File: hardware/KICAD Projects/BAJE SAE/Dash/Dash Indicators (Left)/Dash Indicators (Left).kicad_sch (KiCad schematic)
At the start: 16 parts

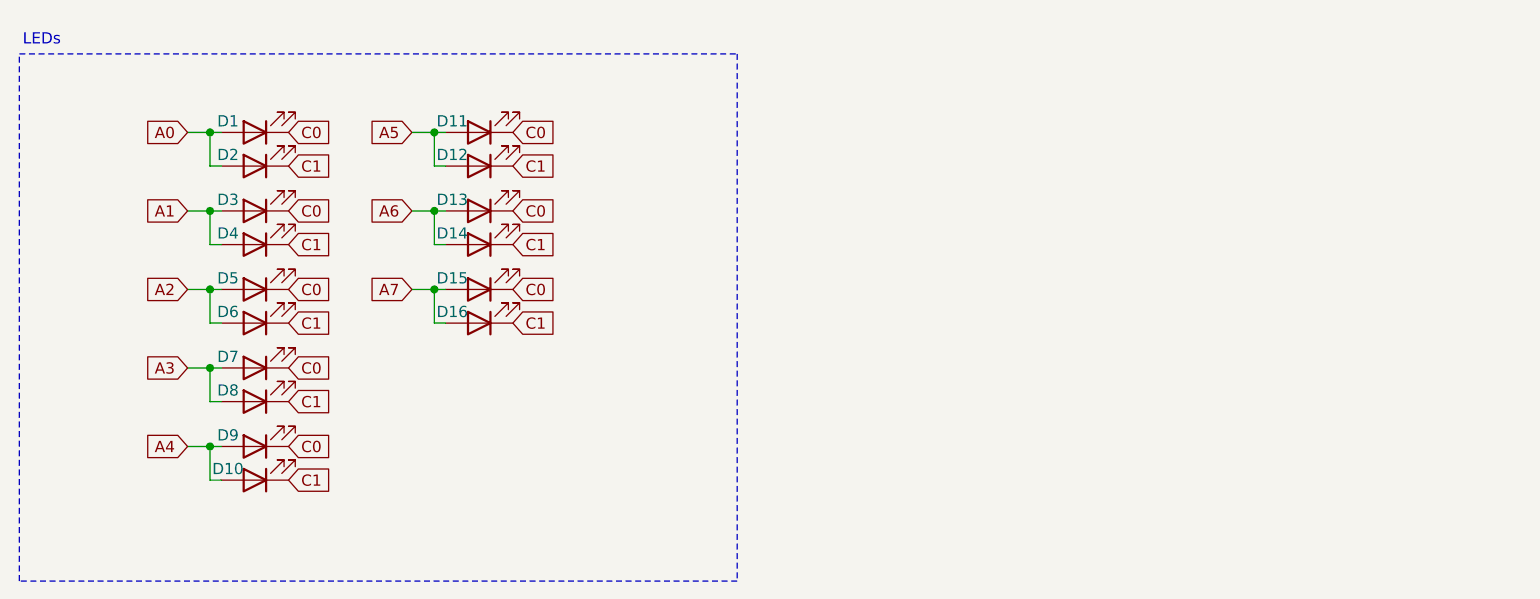
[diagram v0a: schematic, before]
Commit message: dash updates
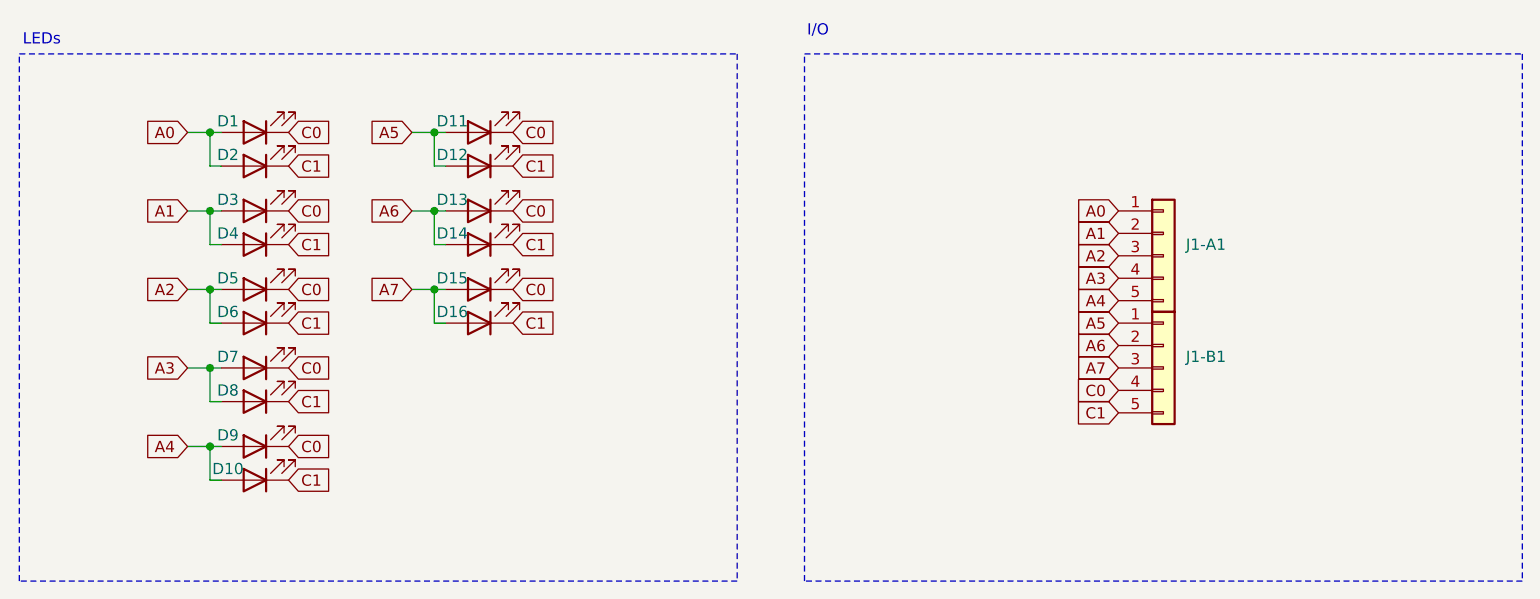
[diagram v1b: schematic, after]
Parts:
- added J1-A1, J1-B1: Conn_01x05, Connector_PinHeader_2.54mm:PinHeader_1x05_P2.54mm_Vertical, symbol Connector_Generic:Conn_01x05
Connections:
- net A0: now also J1-A1.1 (Pin_1)
- net A1: now also J1-A1.2 (Pin_2)
- net A2: now also J1-A1.3 (Pin_3)
- net A3: now also J1-A1.4 (Pin_4)
- net A4: now also J1-A1.5 (Pin_5)
- net A5: now also J1-B1.1 (Pin_1)
- net A6: now also J1-B1.2 (Pin_2)
- net A7: now also J1-B1.3 (Pin_3)
- net C0: now also J1-B1.4 (Pin_4)
- net C1: now also J1-B1.5 (Pin_5)
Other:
- note added: "I/O"
